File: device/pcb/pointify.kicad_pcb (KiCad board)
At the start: 2 copper layers, 14 parts, among them J1 PWM, J2 JTAG, J3 USB_C, U1 XC6206P332MR, U2 STM32F070F6P6, Y1 8MHz

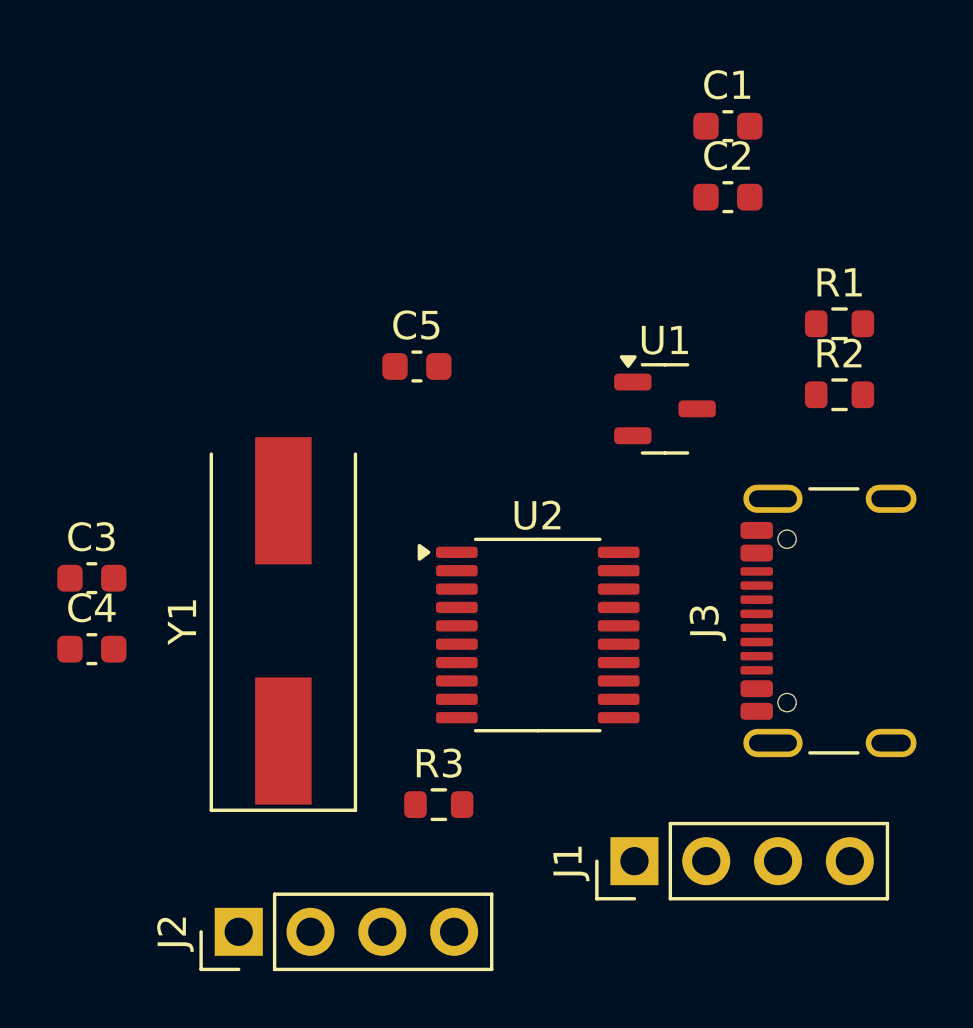
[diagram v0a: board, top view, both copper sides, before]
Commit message: add: complete pcb artwork
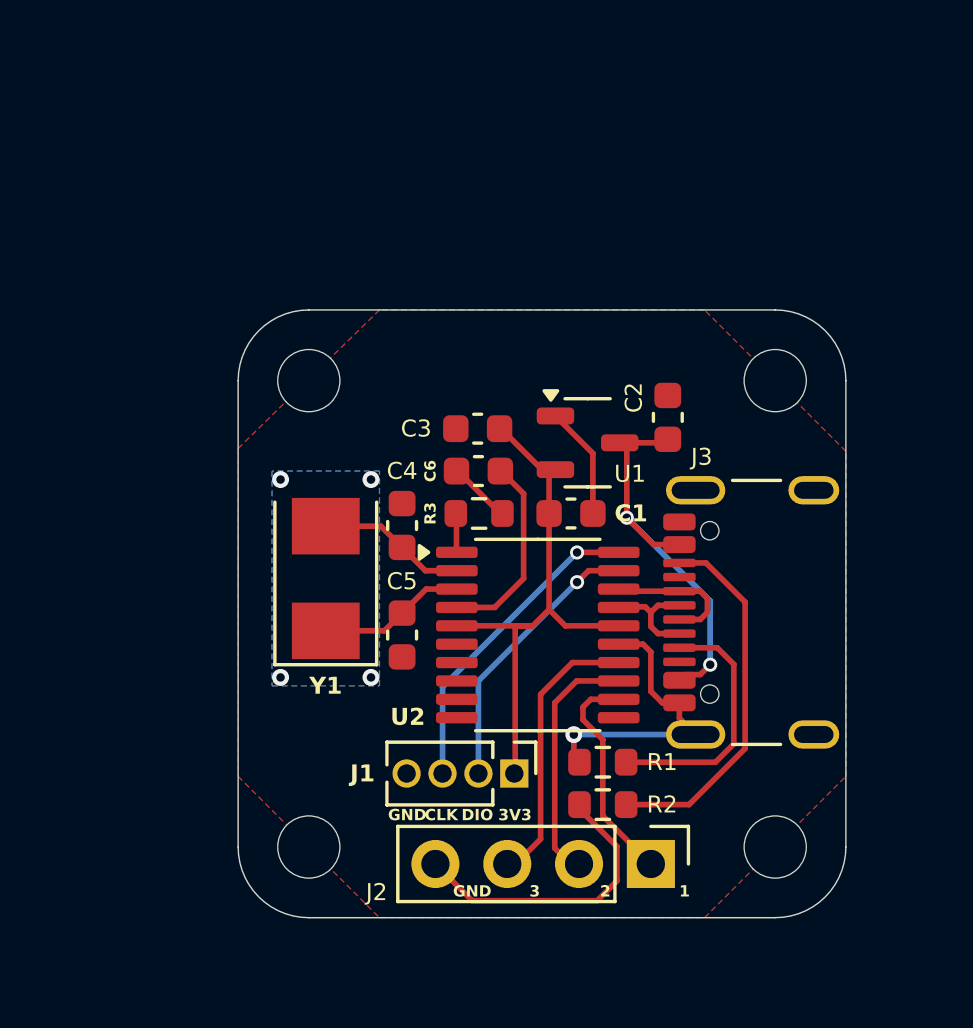
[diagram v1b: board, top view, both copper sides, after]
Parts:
- added C1: 100nF, Capacitor_SMD:C_0603_1608Metric, F.Cu at (131.2, 74.7)
- added G***: LOGO, pcb:luftaquila, B.Cu at (130.0, 78.5)
- added REF**: MountingHole_2.2mm_M2, MountingHole:MountingHole_2.2mm_M2, F.Cu at (138.4, 86.5)
- added REF**: MountingHole_2.2mm_M2, MountingHole:MountingHole_2.2mm_M2, F.Cu at (138.4, 70.0)
- added REF**: MountingHole_2.2mm_M2, MountingHole:MountingHole_2.2mm_M2, F.Cu at (121.9, 86.5)
- added REF**: MountingHole_2.2mm_M2, MountingHole:MountingHole_2.2mm_M2, F.Cu at (121.9, 70.0)
- J1: renamed from J2; footprint Connector_PinHeader_2.54mm:PinHeader_1x04_P2.54mm_Vertical -> Connector_PinHeader_1.27mm:PinHeader_1x04_P1.27mm_Vertical
- Y1: footprint Crystal:Crystal_SMD_HC49-SD -> Crystal:Crystal_SMD_5032-2Pin_5.0x3.2mm
- moved R1 17.6 mm to (132.3, 83.5)
- moved R2 16.7 mm to (132.3, 85.0)
- moved C3 12.1 mm to (127.9, 71.7), turned to 180 degrees
- moved J1 11.2 mm to (129.2, 83.9), turned to -90 degrees
- moved C4 11.1 mm to (125.2, 75.1), turned to 90 degrees
- moved C5 11.0 mm to (125.2, 79.0), turned to -90 degrees
- moved C2 10.5 mm to (134.6, 71.3), turned to 90 degrees
- moved R3 10.4 mm to (127.9, 74.7), turned to 180 degrees
- moved C6 4.29 mm to (127.9, 73.2), turned to 180 degrees
- moved U1 2.99 mm to (131.8, 72.2)
- moved J3 2.75 mm to (138.7, 78.2)
- moved Y1 2.12 mm to (122.5, 77.0)
- moved J2 0.59 mm to (134.0, 87.1), turned to -90 degrees
- renumbered C1 to C2, C2 to C3, C3 to C4, C4 to C5, C5 to C6, J1 to J2
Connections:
- C6 pad 1: BOOT -> NRST
- R3 pad 2: NRST -> BOOT
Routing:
- net GND: track 0.00 -> 27.0 mm, vias 0 -> 5
- net +3V3: track 0.00 -> 19.0 mm
- net +5V: track 0.00 -> 14.0 mm, vias 0 -> 2
- net Net-(J3-CC2): track 0.00 -> 13.1 mm
- net SWCLK: track 0.00 -> 11.4 mm, vias 0 -> 1
- net OUT3: track 0.00 -> 10.0 mm
- net SWDIO: track 0.00 -> 9.96 mm, vias 0 -> 1
- net Net-(J3-CC1): track 0.00 -> 9.06 mm
- net OUT2: track 0.00 -> 8.94 mm
- net OUT1: track 0.00 -> 7.92 mm
- net NRST: track 0.00 -> 6.88 mm
- net OSC_OUT: track 0.00 -> 5.41 mm
- net OSC_IN: track 0.00 -> 5.29 mm
- net USB_DP: track 0.00 -> 4.87 mm
- net USB_DM: track 0.00 -> 3.92 mm
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- added copper zone on B.Cu, net GND
- added copper zone on F.Cu, net GND
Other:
- board outline added: 21.5 x 21.5 mm
- board text added: "1"
- board text added: "2"
- board text added: "3"
- board text added: "3V3"
- board text added: "CLK"
- board text added: "DIO"
- board text added: "GND"
- board text added: "JLCJLCJLCJLC"
